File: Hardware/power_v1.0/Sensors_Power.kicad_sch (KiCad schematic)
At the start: 16 parts, among them J1 Conn_01x02, U1 MP2338GTL-Z

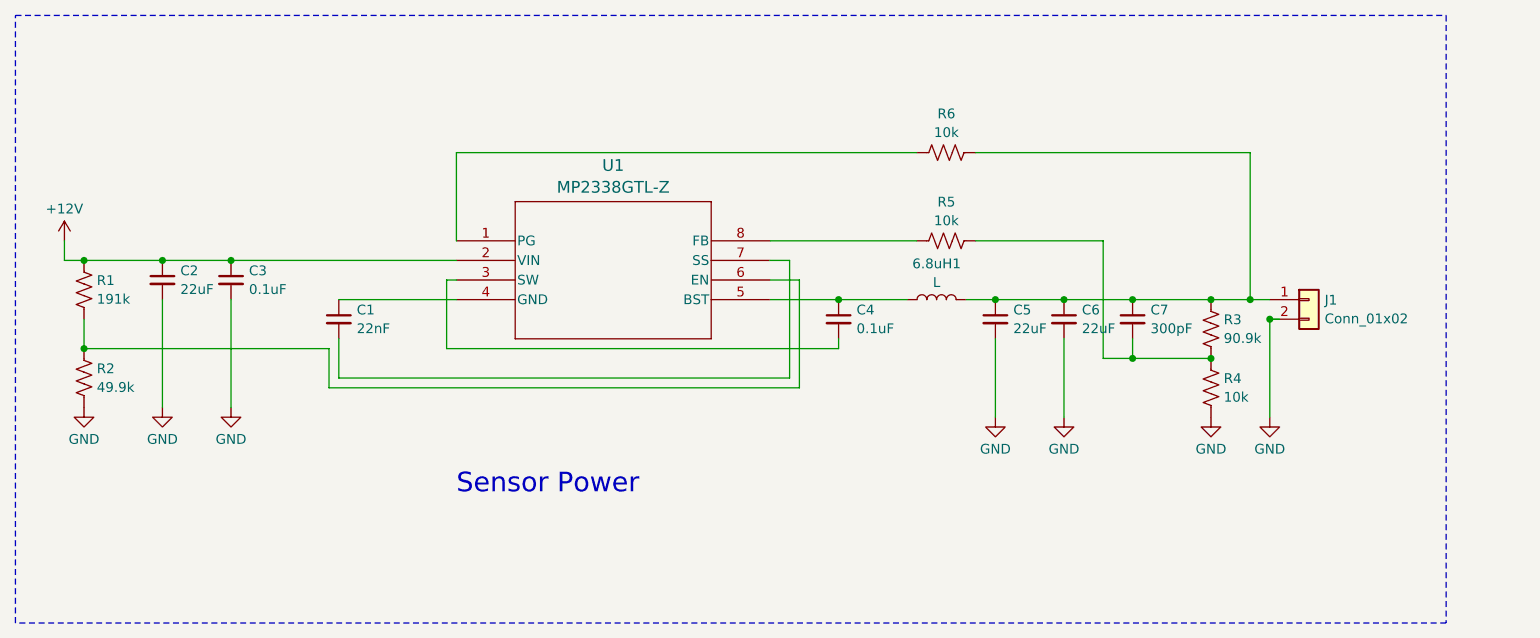
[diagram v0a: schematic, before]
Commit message: almost finished design of power board and working through design of brain board
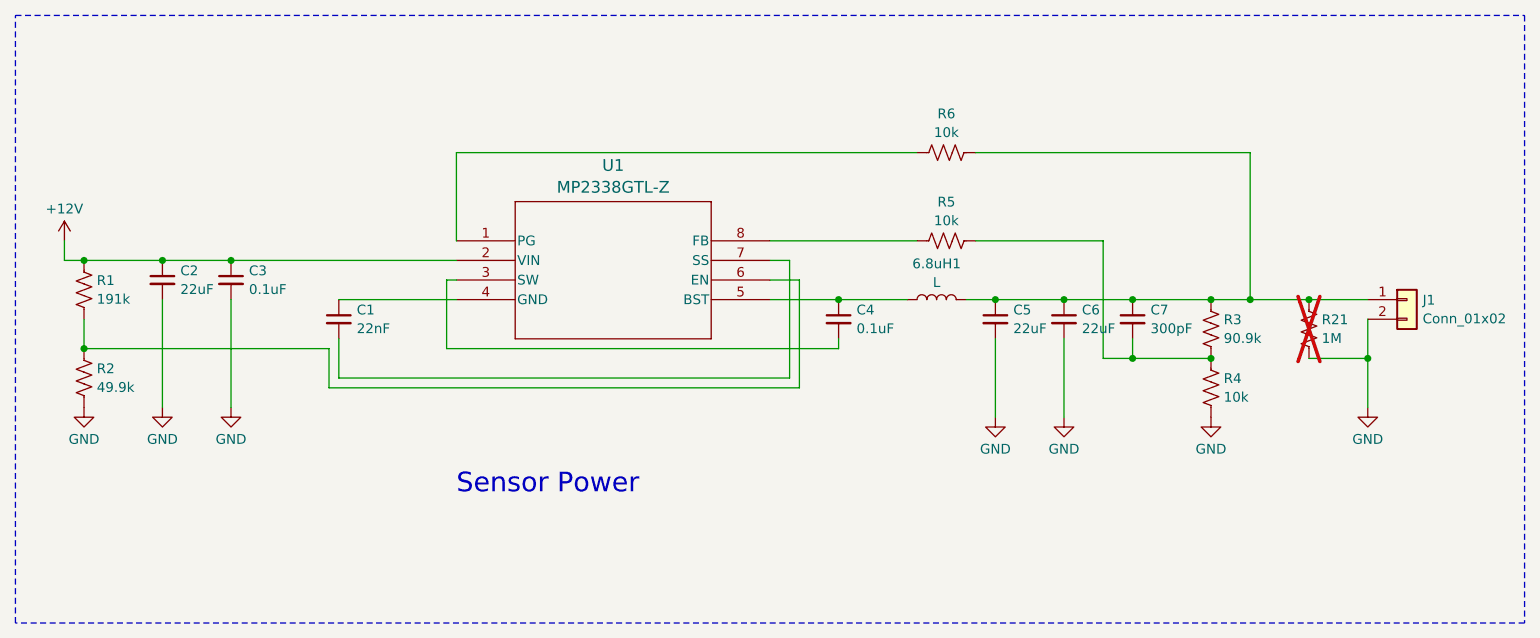
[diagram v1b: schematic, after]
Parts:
- added R21: 1M, symbol Device:R_US
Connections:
- net GND: now also R21.2
- net at 6.8uH1.2, C5.1, C6.1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: now also R21.1
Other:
- moved on the sheet: J1
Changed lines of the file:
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@@
   (junction (at 184.15 95.25) (diameter 0) (color 0 0 0 0)
   )
-  (junction (at 219.71 97.79) (diameter 0) (color 0 0 0 0)
+  (junction (at 232.41 102.87) (diameter 0) (color 0 0 0 0)
   )
   (junction (at 212.09 95.25) (diameter 0) (color 0 0 0 0)
@@
   (junction (at 66.04 90.17) (diameter 0) (color 0 0 0 0)
   )
+  (junction (at 224.79 95.25) (diameter 0) (color 0 0 0 0)
+  )
   (junction (at 217.17 95.25) (diameter 0) (color 0 0 0 0)
   )
@@
     (stroke (width 0) (type default))
   )
+  (wire (pts (xy 224.79 95.25) (xy 232.41 95.25))
+    (stroke (width 0) (type default))
+  )
   (wire (pts (xy 114.3 87.63) (xy 114.3 76.2))
     (stroke (width 0) (type default))
@@
     (stroke (width 0) (type default))
   )
-  (wire (pts (xy 217.17 95.25) (xy 219.71 95.25))
-    (stroke (width 0) (type default))
-  )
-  (wire (pts (xy 219.71 97.79) (xy 220.98 97.79))
+  (wire (pts (xy 217.17 95.25) (xy 224.79 95.25))
     (stroke (width 0) (type default))
   )
@@
     (stroke (width 0) (type default))
   )
-  (wire (pts (xy 219.71 97.79) (xy 219.71 110.49))
+  (wire (pts (xy 232.41 97.79) (xy 232.41 102.87))
     (stroke (width 0) (type default))
   )
@@
     (stroke (width 0) (type default))
   )
+  (wire (pts (xy 224.79 102.87) (xy 232.41 102.87))
+    (stroke (width 0) (type default))
+  )
   (wire (pts (xy 99.06 105.41) (xy 157.48 105.41))
     (stroke (width 0) (type default))
@@
     (stroke (width 0) (type default))
   )
+  (wire (pts (xy 232.41 102.87) (xy 232.41 109.22))
+    (stroke (width 0) (type default))
+  )
   (wire (pts (xy 193.04 100.33) (xy 193.04 110.49))
     (stroke (width 0) (type default))
   )
-  (rectangle (start 57.15 58.42) (end 242.57 137.16)
+  (rectangle (start 57.15 58.42) (end 252.73 137.16)
     (stroke (width 0) (type dash))
     (fill (type none))
@@
     )
   )
-  (symbol (lib_id "power:GND") (at 219.71 110.49 0) (unit 1)
-    (in_bom yes) (on_board yes) (dnp no) (fields_autoplaced)
-    (property "Reference" "#PWR09" (at 219.71 116.84 0)
-      (effects (font (size 1.27 1.27)) hide)
-    )
-    (property "Value" "GND" (at 219.71 114.6231 0)
+  (symbol (lib_id "power:GND") (at 232.41 109.22 0) (unit 1)
+    (in_bom yes) (on_board yes) (dnp no) (fields_autoplaced)
+    (property "Reference" "#PWR09" (at 232.41 115.57 0)
+      (effects (font (size 1.27 1.27)) hide)
+    )
+    (property "Value" "GND" (at 232.41 113.3531 0)
       (effects (font (size 1.27 1.27)))
     )
-    (property "Footprint" "" (at 219.71 110.49 0)
-      (effects (font (size 1.27 1.27)) hide)
-    )
-    (property "Datasheet" "" (at 219.71 110.49 0)
+    (property "Footprint" "" (at 232.41 109.22 0)
+      (effects (font (size 1.27 1.27)) hide)
+    )
+    (property "Datasheet" "" (at 232.41 109.22 0)
       (effects (font (size 1.27 1.27)) hide)
     )
@@
         (path "/1e1b062d-fad0-427c-a622-c5b8a80b5268/e9a765f8-cea6-440c-a615-75e1b7717a8f"
           (reference "#PWR09") (unit 1)
+        )
+      )
+    )
+  )
+  (symbol (lib_id "Device:R_US") (at 224.79 99.06 0) (unit 1)
+    (in_bom yes) (on_board yes) (dnp yes) (fields_autoplaced)
+    (property "Reference" "R21" (at 226.441 97.8479 0)
+      (effects (font (size 1.27 1.27)) (justify left))
+    )
+    (property "Value" "1M" (at 226.441 100.2721 0)
+      (effects (font (size 1.27 1.27)) (justify left))
+    )
+    (property "Footprint" "" (at 225.806 99.314 90)
+      (effects (font (size 1.27 1.27)) hide)
+    )
+    (property "Datasheet" "~" (at 224.79 99.06 0)
+      (effects (font (size 1.27 1.27)) hide)
+    )
+    (pin "1")
+    (pin "2")
+    (instances
+      (project "power_v1.0"
+        (path "/1e1b062d-fad0-427c-a622-c5b8a80b5268/e9a765f8-cea6-440c-a615-75e1b7717a8f"
+          (reference "R21") (unit 1)
         )
       )
@@
     )
   )
-  (symbol (lib_id "Connector_Generic:Conn_01x02") (at 224.79 95.25 0) (unit 1)
-    (in_bom yes) (on_board yes) (dnp no) (fields_autoplaced)
-    (property "Reference" "J1" (at 226.822 95.3079 0)
-      (effects (font (size 1.27 1.27)) (justify left))
-    )
-    (property "Value" "Conn_01x02" (at 226.822 97.7321 0)
-      (effects (font (size 1.27 1.27)) (justify left))
-    )
-    (property "Footprint" "" (at 224.79 95.25 0)
-      (effects (font (size 1.27 1.27)) hide)
-    )
-    (property "Datasheet" "~" (at 224.79 95.25 0)
-      (effects (font (size 1.27 1.27)) hide)
-    )
+  (symbol (lib_id "Connector_Generic:Conn_01x02") (at 237.49 95.25 0) (unit 1)
+    (in_bom yes) (on_board yes) (dnp no) (fields_autoplaced)
+    (property "Reference" "J1" (at 239.522 95.3079 0)
+      (effects (font (size 1.27 1.27)) (justify left))
+    )
+    (property "Value" "Conn_01x02" (at 239.522 97.7321 0)
+      (effects (font (size 1.27 1.27)) (justify left))
+    )
+    (property "Footprint" "" (at 237.49 95.25 0)
+      (effects (font (size 1.27 1.27)) hide)
+    )
+    (property "Datasheet" "~" (at 237.49 95.25 0)
+      (effects (font (size 1.27 1.27)) hide)
+    )
